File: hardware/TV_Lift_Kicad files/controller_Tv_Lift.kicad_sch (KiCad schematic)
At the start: 102 parts, among them J1 socket LAN8720a, J10 1844210, J11 1844223, J12 C5360899, J2 1836189, J3 1844223, J4 1844210, J5 1844223, J6 1844223, J7 1844236, J8 C5360899, J9 1844210, Q2 MMBT3906, SW1 TS-1187A-BAB, SW2 TS-1187A-BAB, SW3 TS-1187A-BAB, SW4 TS-1187A-BAB, U1 MAX3232, U10 VNH5019ATR-E, U2 TSOP32S40F, U3 SN65HVD230, U4 ESP32-WROOM-32, U5 LM2596S-5, U6 AMS1117-3.3, U7 PC817, U8 PC817, U9 b0505s-1we

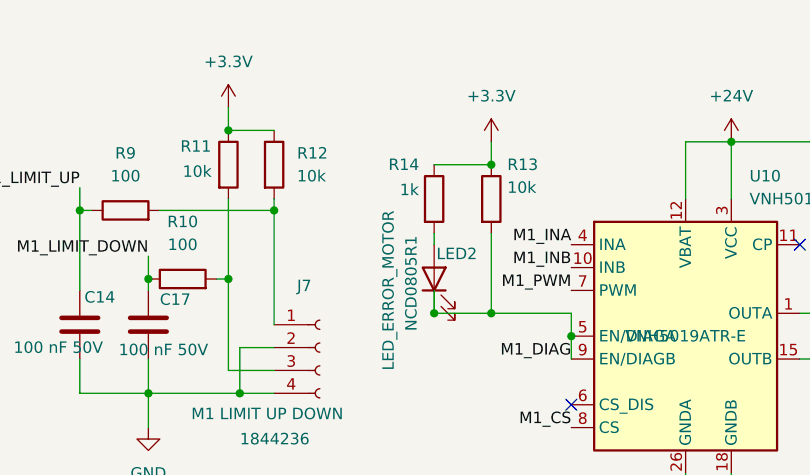
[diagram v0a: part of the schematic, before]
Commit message: fix  overcurrent
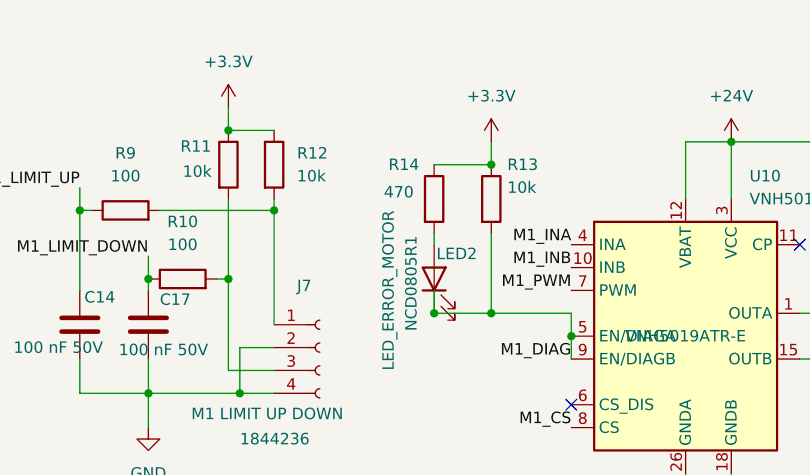
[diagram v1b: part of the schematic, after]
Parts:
- R14: value 1k -> 470
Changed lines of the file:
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@@
 			)
 		)
-		(property "Value" "1k"
-			(at 196.85 32.004 0)
+		(property "Value" "470"
+			(at 195.072 32.258 0)
 			(show_name no)
 			(do_not_autoplace no)
